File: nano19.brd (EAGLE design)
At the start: 40.6 x 20.3 mm, 5 parts, among them J3 JUMPER-JP-2, J4 JUMPER-JP-2

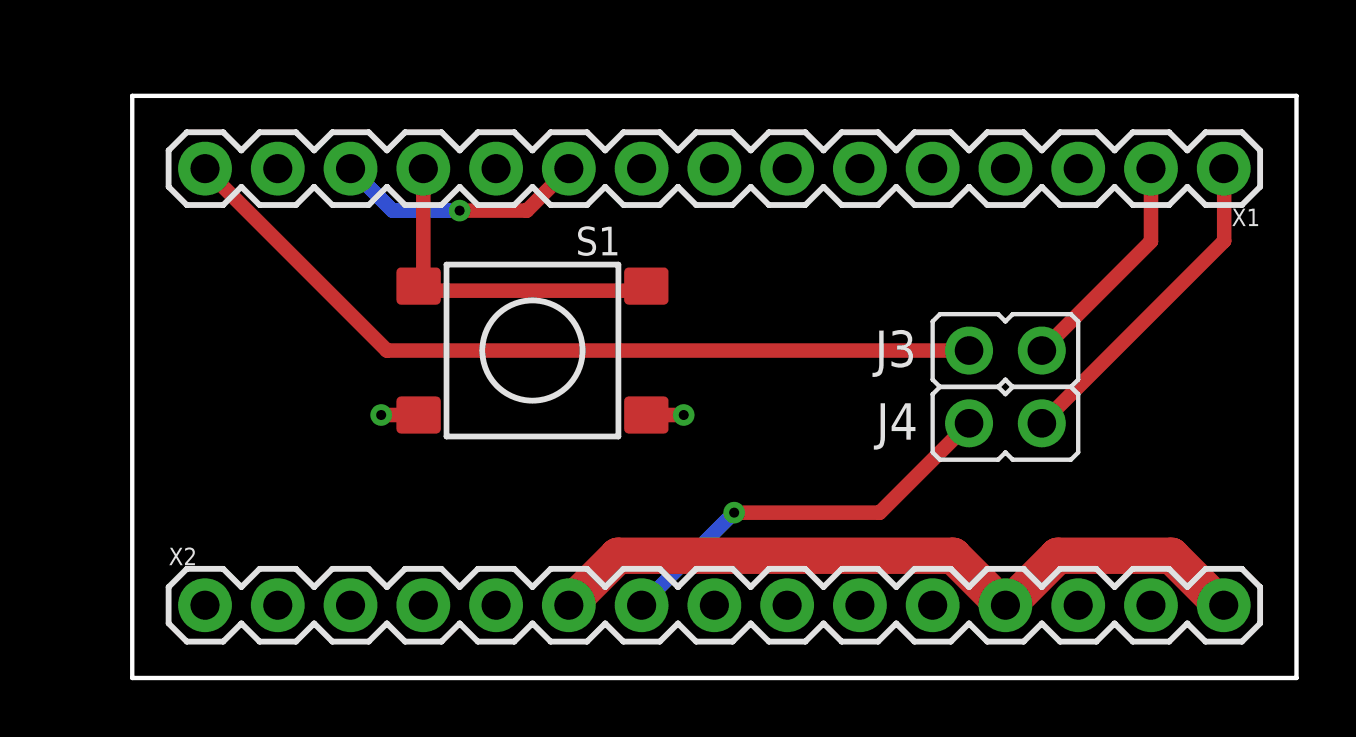
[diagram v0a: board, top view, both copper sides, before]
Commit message: - nano.brd (Routing + Layout + Text)
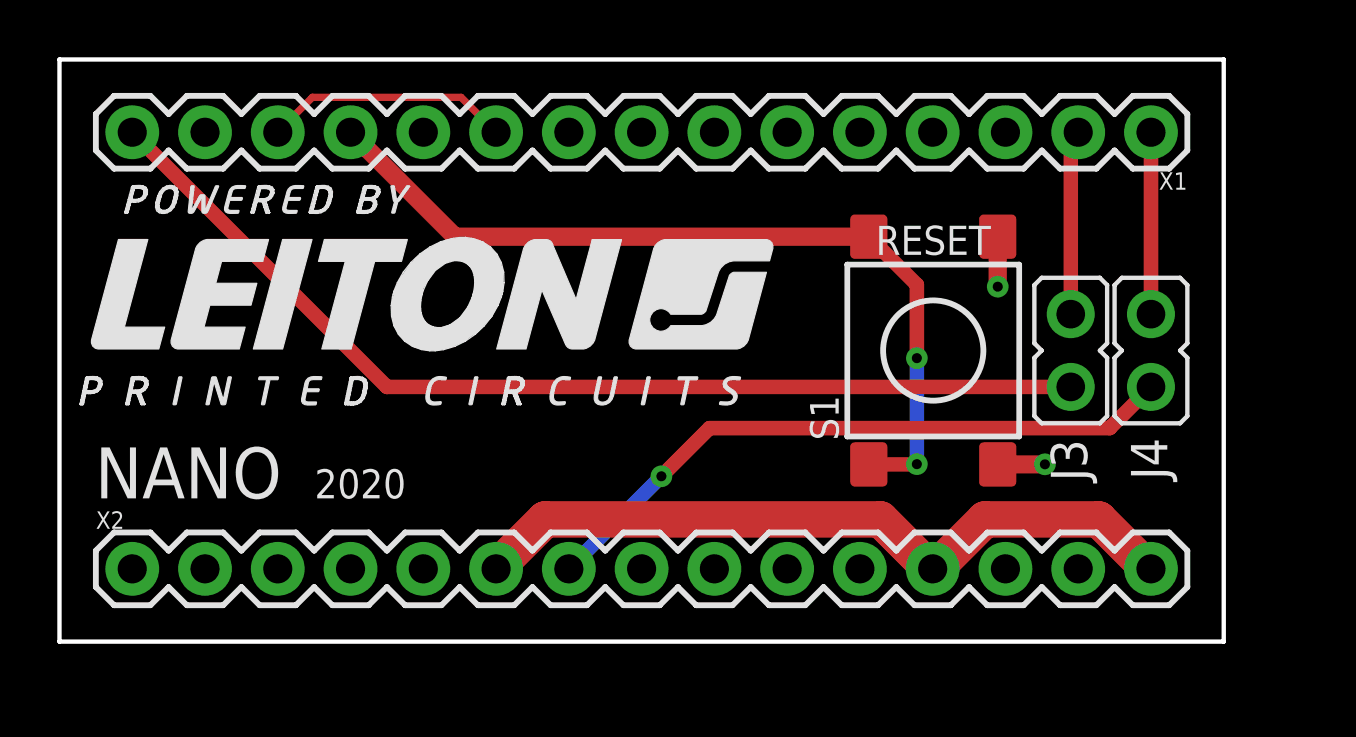
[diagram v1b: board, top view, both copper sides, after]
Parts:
- moved S1 14.0 mm to (30.5, 10.2), turned to 270 degrees
- moved J4 5.68 mm to (38.1, 10.2), turned to 180 degrees
- moved X2 2.84 mm to (2.54, 2.54)
- moved X1 2.84 mm to (38.1, 17.8)
- moved J3 2.28 mm to (35.3, 10.2), turned to 180 degrees
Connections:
- removed net LED: X1.14
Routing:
- net ARD-RESET: track 12.3 -> 29.9 mm, vias 0 -> 2
- net RX: track 14.1 -> 23.0 mm
- net TX: track 29.3 -> 36.4 mm
- net N$2: track 11.5 -> 6.35 mm
- net N$1: track 7.93 -> 6.46 mm
- net GND: track 2.61 -> 3.40 mm
- net ARD-INTERRUPT: track 8.83 -> 8.64 mm, vias 1 -> 0
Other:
- board text added: "2020"
- board text added: "NANO"
- board text added: "RESET"

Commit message: - brd (Labeling)
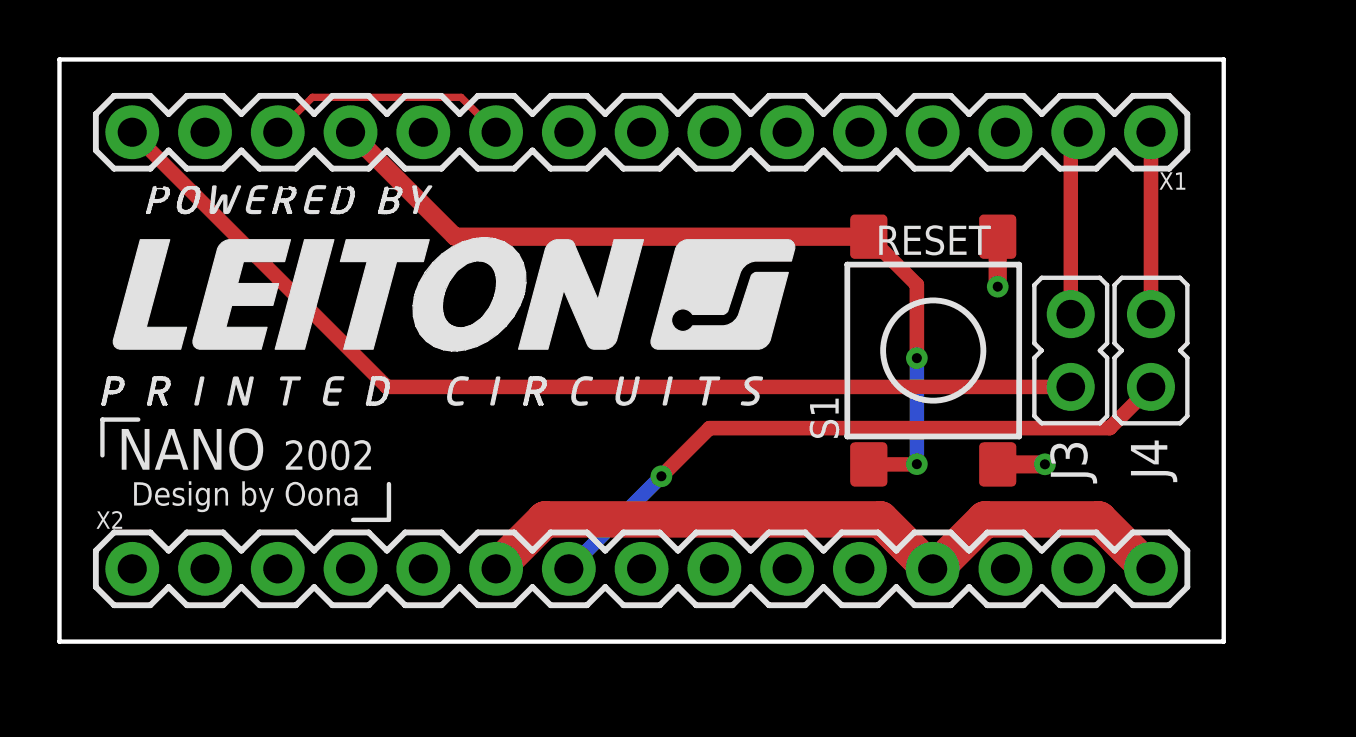
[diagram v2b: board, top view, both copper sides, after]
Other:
- board text added: "2002"
- board text added: "Design by Oona"
- board text removed: "2020"
